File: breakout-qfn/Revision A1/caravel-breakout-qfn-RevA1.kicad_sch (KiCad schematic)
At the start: 14 parts, among them CON1 REF-182665-01, CON2 REF-182665-01, CON3 73251-1352, U1 Caravel, U2 TLV73318PDBV

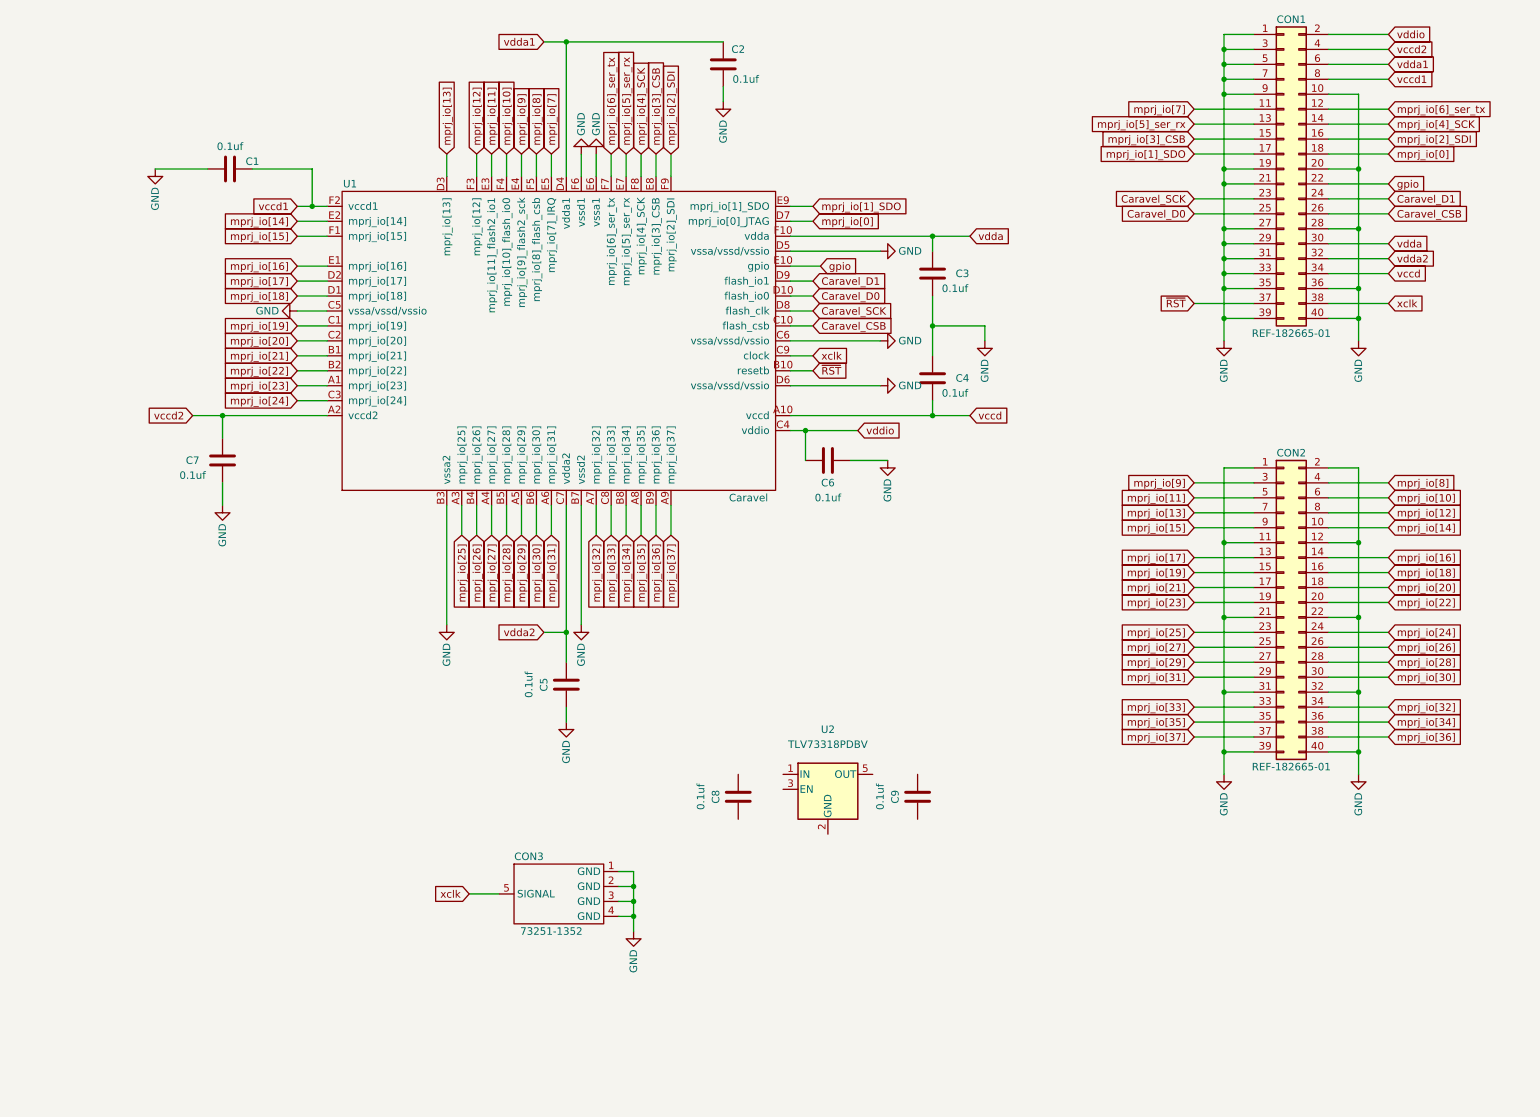
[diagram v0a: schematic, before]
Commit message: WIP checkin for comments
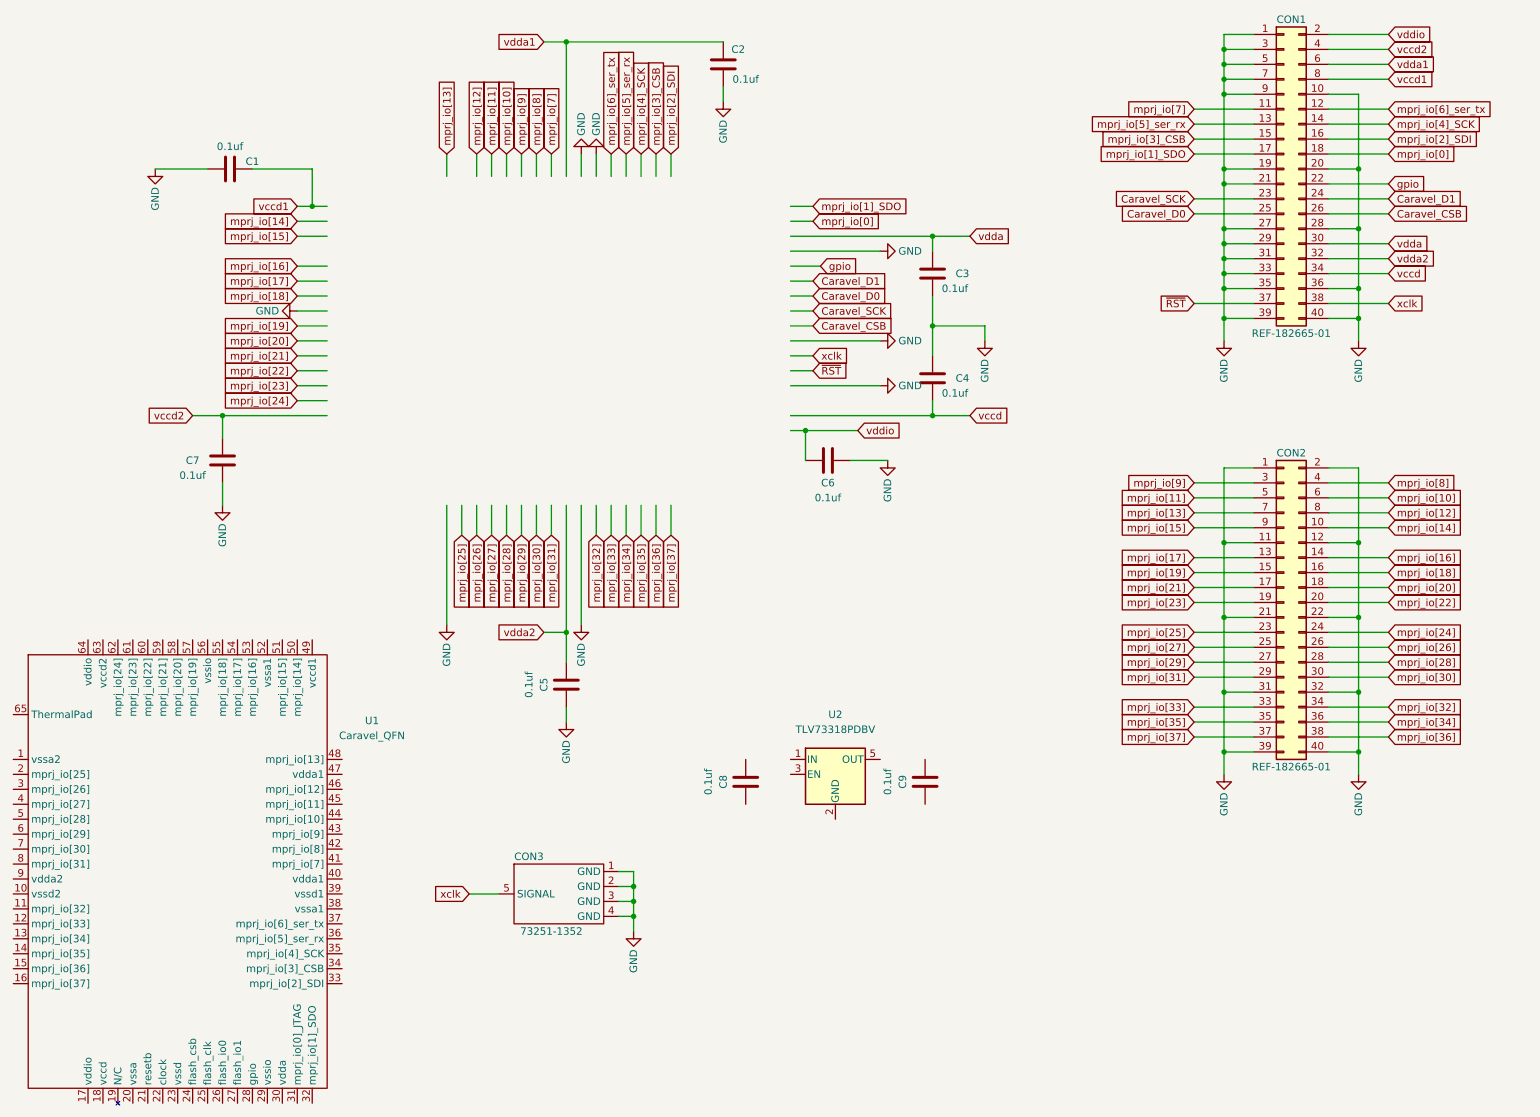
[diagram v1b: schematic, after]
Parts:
- removed U1: Caravel, ok-chips:Caravel_WLCSP, symbol ok-chips:Caravel_WLCSP
- added U1: Caravel_QFN, Package_DFN_QFN:QFN-64-1EP_9x9mm_P0.5mm_EP7.65x7.65mm, symbol ok-chips:Caravel_QFN
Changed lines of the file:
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@@
     )
-  )
-  (symbol (lib_id "ok-chips:Caravel_WLCSP") (at 93.98 82.55 90) (unit 1)
-    (in_bom yes) (on_board yes)
-    (property "Reference" "U1" (id 0) (at 64.77 54.61 90)
-      (effects (font (size 1.27 1.27)) (justify left))
-    )
-    (property "Value" "Caravel" (id 1) (at 134.62 107.95 90)
-      (effects (font (size 1.27 1.27)) (justify left))
-    )
-    (property "Footprint" "ok-chips:Caravel_WLCSP" (id 2) (at 137.16 54.61 0)
-      (effects (font (size 1.27 1.27)) (justify left) hide)
-    )
-    (property "Datasheet" "" (id 3) (at 93.98 82.55 0)
-      (effects (font (size 1.27 1.27)) hide)
-    )
-    (property "LibSource" "https://github.com/efabless/caravel_board/blob/84c2a618c3ccb63b4e827d80adff53c441349ad6/hardware/symbols/Caravel_board.kicad_sym" (id 4) (at 139.7 54.61 0)
-      (effects (font (size 1.27 1.27)) (justify left) hide)
-    )
-    (pin "A1")
-    (pin "A10")
-    (pin "A2")
-    (pin "A3")
-    (pin "A4")
-    (pin "A5")
-    (pin "A6")
-    (pin "A7")
-    (pin "A8")
-    (pin "A9")
-    (pin "B1")
-    (pin "B10")
-    (pin "B2")
-    (pin "B3")
-    (pin "B4")
-    (pin "B5")
-    (pin "B6")
-    (pin "B7")
-    (pin "B8")
-    (pin "B9")
-    (pin "C1")
-    (pin "C10")
-    (pin "C2")
-    (pin "C3")
-    (pin "C4")
-    (pin "C5")
-    (pin "C6")
-    (pin "C7")
-    (pin "C8")
-    (pin "C9")
-    (pin "D1")
-    (pin "D10")
-    (pin "D2")
-    (pin "D3")
-    (pin "D4")
-    (pin "D5")
-    (pin "D6")
-    (pin "D7")
-    (pin "D8")
-    (pin "D9")
-    (pin "E1")
-    (pin "E10")
-    (pin "E2")
-    (pin "E3")
-    (pin "E4")
-    (pin "E5")
-    (pin "E6")
-    (pin "E7")
-    (pin "E8")
-    (pin "E9")
-    (pin "F1")
-    (pin "F10")
-    (pin "F2")
-    (pin "F3")
-    (pin "F4")
-    (pin "F5")
-    (pin "F6")
-    (pin "F7")
-    (pin "F8")
-    (pin "F9")
   )
   (symbol (lib_id "Device:C") (at 162.56 69.85 0) (unit 1)
@@
     )
     (pin "1")
-  )
-  (symbol (lib_id "Regulator_Linear:TLV73318PDBV") (at 144.78 157.48 0) (unit 1)
-    (in_bom yes) (on_board yes) (fields_autoplaced)
-    (property "Reference" "U2" (id 0) (at 144.78 147.32 0))
-    (property "Value" "TLV73318PDBV" (id 1) (at 144.78 149.86 0))
-    (property "Footprint" "Package_TO_SOT_SMD:SOT-23-5" (id 2) (at 144.78 149.225 0)
-      (effects (font (size 1.27 1.27) italic) hide)
-    )
-    (property "Datasheet" "http://www.ti.com/lit/ds/symlink/tlv733p.pdf" (id 3) (at 144.78 157.48 0)
-      (effects (font (size 1.27 1.27)) hide)
-    )
-    (pin "1")
-    (pin "2")
-    (pin "3")
-    (pin "4")
-    (pin "5")
   )
   (symbol (lib_id "Connector_Generic:Conn_02x20_Odd_Even") (at 222.25 52.07 0) (unit 1)
@@
     (pin "9")
   )
+  (symbol (lib_id "Device:C") (at 161.29 156.21 180) (unit 1)
+    (in_bom yes) (on_board yes)
+    (property "Reference" "C9" (id 0) (at 157.48 156.21 90))
+    (property "Value" "0.1uf" (id 1) (at 154.94 156.21 90))
+    (property "Footprint" "Capacitor_SMD:C_0603_1608Metric" (id 2) (at 160.3248 152.4 0)
+      (effects (font (size 1.27 1.27)) hide)
+    )
+    (property "Datasheet" "~" (id 3) (at 161.29 156.21 0)
+      (effects (font (size 1.27 1.27)) hide)
+    )
+    (pin "1")
+    (pin "2")
+  )
+  (symbol (lib_id "Regulator_Linear:TLV73318PDBV") (at 146.05 154.94 0) (unit 1)
+    (in_bom yes) (on_board yes) (fields_autoplaced)
+    (property "Reference" "U2" (id 0) (at 146.05 144.78 0))
+    (property "Value" "TLV73318PDBV" (id 1) (at 146.05 147.32 0))
+    (property "Footprint" "Package_TO_SOT_SMD:SOT-23-5" (id 2) (at 146.05 146.685 0)
+      (effects (font (size 1.27 1.27) italic) hide)
+    )
+    (property "Datasheet" "http://www.ti.com/lit/ds/symlink/tlv733p.pdf" (id 3) (at 146.05 154.94 0)
+      (effects (font (size 1.27 1.27)) hide)
+    )
+    (pin "1")
+    (pin "2")
+    (pin "3")
+    (pin "4")
+    (pin "5")
+  )
   (symbol (lib_id "power:GND") (at 234.95 81.28 0) (unit 1)
     (in_bom yes) (on_board yes)
@@
     (pin "1")
   )
+  (symbol (lib_id "ok-chips:Caravel_QFN") (at 35.56 175.26 0) (unit 1)
+    (in_bom yes) (on_board yes) (fields_autoplaced)
+    (property "Reference" "U1" (id 0) (at 67.31 145.8212 0))
+    (property "Value" "Caravel_QFN" (id 1) (at 67.31 148.3612 0))
+    (property "Footprint" "Package_DFN_QFN:QFN-64-1EP_9x9mm_P0.5mm_EP7.65x7.65mm" (id 2) (at 60.96 209.55 0)
+      (effects (font (size 1.27 1.27)) (justify left) hide)
+    )
+    (property "Datasheet" "" (id 3) (at 35.56 175.26 0)
+      (effects (font (size 1.27 1.27)) hide)
+    )
+    (property "LibSource" "https://github.com/efabless/caravel_board/blob/84c2a618c3ccb63b4e827d80adff53c441349ad6/hardware/symbols/Caravel_board.kicad_sym" (id 4) (at 60.96 212.09 0)
+      (effects (font (size 1.27 1.27)) (justify left) hide)
+    )
+    (pin "1")
+    (pin "10")
+    (pin "11")
+    (pin "12")
+    (pin "13")
+    (pin "14")
+    (pin "15")
+    (pin "16")
+    (pin "17")
+    (pin "18")
+    (pin "19")
+    (pin "2")
+    (pin "20")
+    (pin "21")
+    (pin "22")
+    (pin "23")
+    (pin "24")
+    (pin "25")
+    (pin "26")
+    (pin "27")
+    (pin "28")
+    (pin "29")
+    (pin "3")
+    (pin "30")
+    (pin "31")
+    (pin "32")
+    (pin "33")
+    (pin "34")
+    (pin "35")
+    (pin "36")
+    (pin "37")
+    (pin "38")
+    (pin "39")
+    (pin "4")
+    (pin "40")
+    (pin "41")
+    (pin "42")
+    (pin "43")
+    (pin "44")
+    (pin "45")
+    (pin "46")
+    (pin "47")
+    (pin "48")
+    (pin "49")
+    (pin "5")
+    (pin "50")
+    (pin "51")
+    (pin "52")
+    (pin "53")
+    (pin "54")
+    (pin "55")
+    (pin "56")
+    (pin "57")
+    (pin "58")
+    (pin "59")
+    (pin "6")
+    (pin "60")
+    (pin "61")
+    (pin "62")
+    (pin "63")
+    (pin "64")
+    (pin "65")
+    (pin "7")
+    (pin "8")
+    (pin "9")
+  )
   (symbol (lib_id "power:GND") (at 212.09 81.28 0) (unit 1)
     (in_bom yes) (on_board yes)
@@
     (pin "1")
   )
-  (symbol (lib_id "Device:C") (at 129.54 158.75 180) (unit 1)
-    (in_bom yes) (on_board yes)
-    (property "Reference" "C8" (id 0) (at 125.73 158.75 90))
-    (property "Value" "0.1uf" (id 1) (at 123.19 158.75 90))
-    (property "Footprint" "Capacitor_SMD:C_0603_1608Metric" (id 2) (at 128.5748 154.94 0)
-      (effects (font (size 1.27 1.27)) hide)
-    )
-    (property "Datasheet" "~" (id 3) (at 129.54 158.75 0)
-      (effects (font (size 1.27 1.27)) hide)
-    )
-    (pin "1")
-    (pin "2")
-  )
   (symbol (lib_id "power:GND") (at 212.09 154.94 0) (unit 1)
     (in_bom yes) (on_board yes)
@@
     (pin "1")
   )
-  (symbol (lib_id "Device:C") (at 160.02 158.75 180) (unit 1)
-    (in_bom yes) (on_board yes)
-    (property "Reference" "C9" (id 0) (at 156.21 158.75 90))
-    (property "Value" "0.1uf" (id 1) (at 153.67 158.75 90))
-    (property "Footprint" "Capacitor_SMD:C_0603_1608Metric" (id 2) (at 159.0548 154.94 0)
-      (effects (font (size 1.27 1.27)) hide)
-    )
-    (property "Datasheet" "~" (id 3) (at 160.02 158.75 0)
+  (symbol (lib_id "Device:C") (at 130.81 156.21 180) (unit 1)
+    (in_bom yes) (on_board yes)
+    (property "Reference" "C8" (id 0) (at 127 156.21 90))
+    (property "Value" "0.1uf" (id 1) (at 124.46 156.21 90))
+    (property "Footprint" "Capacitor_SMD:C_0603_1608Metric" (id 2) (at 129.8448 152.4 0)
+      (effects (font (size 1.27 1.27)) hide)
+    )
+    (property "Datasheet" "~" (id 3) (at 130.81 156.21 0)
       (effects (font (size 1.27 1.27)) hide)
     )
@@
       (reference "C7") (unit 1) (value "0.1uf") (footprint "Capacitor_SMD:C_0402_1005Metric")
     )
-    (path "/748e673c-62ba-48f2-8c93-fcf00774af87"
+    (path "/a1f5d155-7c5b-450f-835a-1beaa84985c2"
       (reference "C8") (unit 1) (value "0.1uf") (footprint "Capacitor_SMD:C_0603_1608Metric")
     )
-    (path "/9c14b6d3-b2f0-4fdc-9232-d4338971c346"
+    (path "/490fa7a0-dc17-4ffe-be30-513cc3f5aca8"
       (reference "C9") (unit 1) (value "0.1uf") (footprint "Capacitor_SMD:C_0603_1608Metric")
     )
@@
       (reference "CON3") (unit 1) (value "73251-1352") (footprint "ok-connectors:TE_5-1814832-2")
     )
-    (path "/00000000-0000-0000-0000-0000612e097b"
-      (reference "U1") (unit 1) (value "Caravel") (footprint "ok-chips:Caravel_WLCSP")
-    )
-    (path "/0d29bb03-4b1f-4213-ba3c-74ea953f1fc4"
+    (path "/629c3e8d-0778-4ca7-bedf-2cc0e61e7e2f"
+      (reference "U1") (unit 1) (value "Caravel_QFN") (footprint "Package_DFN_QFN:QFN-64-1EP_9x9mm_P0.5mm_EP7.65x7.65mm")
+    )
+    (path "/54c9bf1d-870a-4c32-88f6-52ae382a86f1"
       (reference "U2") (unit 1) (value "TLV73318PDBV") (footprint "Package_TO_SOT_SMD:SOT-23-5")
     )
